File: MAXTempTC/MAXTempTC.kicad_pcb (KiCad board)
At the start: 2 copper layers, 15.6 x 29.1 mm, 12 parts, among them J1 1, J2 2, P5 OUTPUT, P6 INPUT, U3 MAX31855, U4 MAX31855

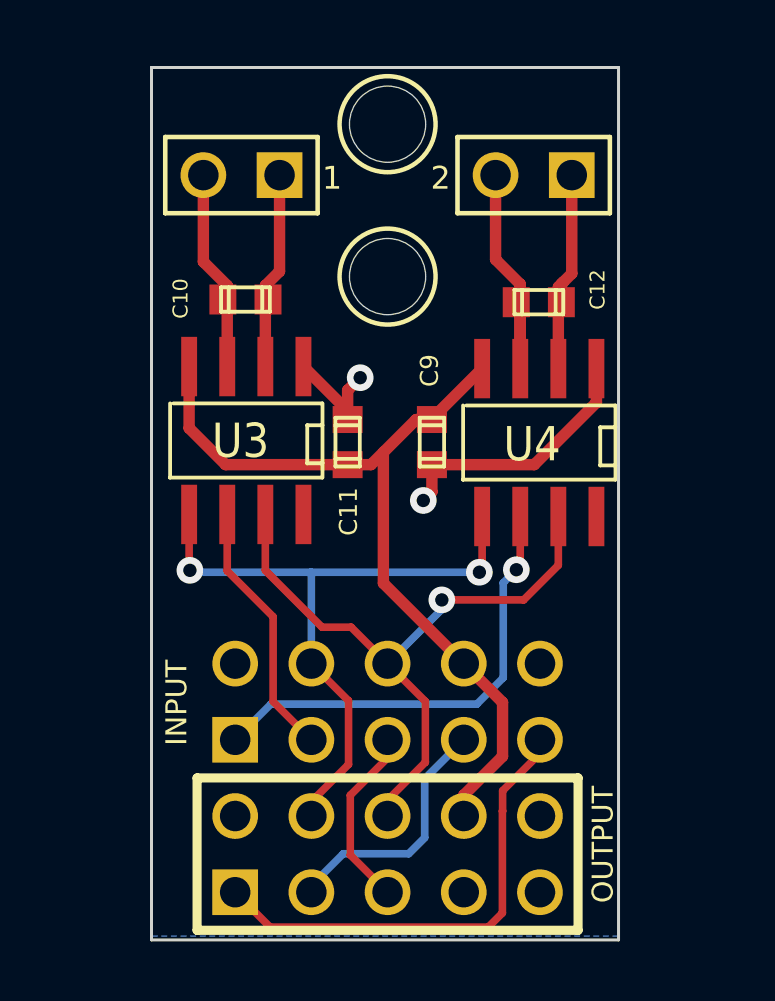
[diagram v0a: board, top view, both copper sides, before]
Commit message: Updated v1.1 source files
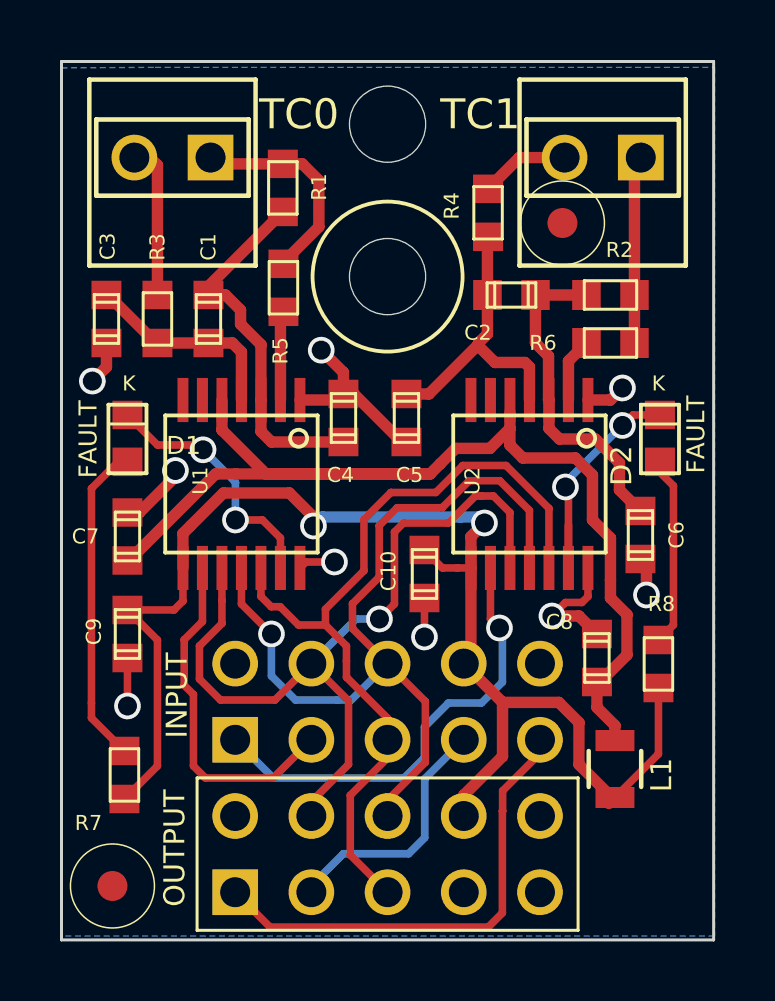
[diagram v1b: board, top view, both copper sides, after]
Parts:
- removed C11: 0.1u, c_0603
- removed C12: 0.01u, c_0603
- removed Mount (x2): VAL**, Mount
- removed U3, U4: MAX31855, MAX81855
- added C1: 0.1u, complib:C_0603, F.Cu at (43.4, 38.7)
- added C2: 0.1u, complib:C_0603, F.Cu at (53.5, 37.9)
- added C3: 0.01u, complib:C_0603, F.Cu at (40.0, 38.7)
- added C4: 0.01u, complib:C_0603, F.Cu at (47.9, 42.0)
- added C5: 0.01u, complib:C_0603, F.Cu at (50.0, 42.0)
- added C6: 0.01u, complib:C_0603, F.Cu at (57.8, 45.9)
- added C7: 0.1u, complib:C_0603, F.Cu at (40.7, 45.9)
- added C8: 0.1u, complib:C_0603, F.Cu at (56.4, 50.0)
- added D1: FAULT, complib:D_0603, F.Cu at (40.7, 42.7)
- added D2: FAULT, complib:D_0603, F.Cu at (58.5, 42.7)
- added G***: LOGO, complib:LOGO_Duet3dCompatible_xs, B.Cu at (42.8, 43.0)
- added L1: 100 µH, complib:R_0805, F.Cu at (57.0, 53.7)
- added M3: FID, complib:Fiducial_1mm_Dia_2.54mm_Outer_CopperTop, F.Cu at (40.2, 57.6)
- added M3: FID, complib:Fiducial_1mm_Dia_2.54mm_Outer_CopperTop, F.Cu at (55.2, 35.5)
- added R1: 100R, complib:R_0603, F.Cu at (45.9, 34.3)
- added R2: 100R, complib:R_0603, F.Cu at (56.8, 37.9)
- added R3: 100R, complib:R_0603, F.Cu at (41.7, 38.7)
- added R4: 100R, complib:R_0603, F.Cu at (52.8, 35.1)
- added R5: 100R, complib:R_0603, F.Cu at (45.9, 37.6)
- added R6: 100R, complib:R_0603, F.Cu at (56.8, 39.5)
- added R7: 330R, complib:R_0603, F.Cu at (40.6, 53.9)
- added R8: 330R, complib:R_0603, F.Cu at (58.4, 50.2)
- added U1: MAX31856, complib:TSSOP-14, F.Cu at (44.5, 44.2)
- added U2: MAX31856, complib:TSSOP-14, F.Cu at (54.1, 44.2)
- C10: value 0.01u -> 0.1u; footprint c_0603 -> complib:C_0603
- C9: footprint c_0603 -> complib:C_0603
- J1: value 1 -> ThermC1; footprint PIN_ARRAY_2X1 -> complib:PIN_ARRAY_2X1
- J2: value 2 -> ThermC2; footprint PIN_ARRAY_2X1 -> complib:PIN_ARRAY_2X1
- P5: footprint PIN_ARRAY_5x2 -> MAX_TEMP_DB
- P6: footprint PIN_ARRAY_5x2 -> complib:MAX_TEMP_DB_inv; moved to B.Cu
- moved C9 12.0 mm to (40.7, 49.2), turned to 270 degrees
- moved C10 10.9 mm to (50.6, 47.2), turned to 270 degrees
- moved J1 2.37 mm to (42.2, 33.3)
- moved J2 2.37 mm to (56.6, 33.3)
- turned P6 to 180 degrees
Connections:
- C10 pad 1: TC+_A -> AGND
- C10 pad 2: TC-_A -> 3.3V
- C9 pad 1: 3.3V -> AGND
- C9 pad 2: GND -> 3.3V
- P5 pad 2: GND -> AGND
- P6 pad 2: GND -> AGND
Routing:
- net AVDD: track 0.00 -> 37.5 mm
- net MOSI: track 6.13 -> 28.4 mm
- net AGND: track 0.00 -> 20.8 mm, vias 0 -> 9
- net 3.3V: track 28.0 -> 46.2 mm, vias 0 -> 2
- net GND: track 12.7 -> 0.00 mm, vias 2 -> 0
- net Net-(C1-Pad2): track 0.00 -> 12.3 mm
- net Net-(C2-Pad2): track 0.00 -> 11.1 mm
- net Net-(D1-Pad1): track 0.00 -> 10.8 mm
- net Net-(C2-Pad1): track 0.00 -> 10.0 mm
- net Net-(D1-Pad2): track 0.00 -> 8.54 mm, vias 0 -> 2
- net Net-(D2-Pad2): track 0.00 -> 8.42 mm, vias 0 -> 2
- net Net-(C1-Pad1): track 0.00 -> 6.89 mm
- net Net-(D2-Pad1): track 0.00 -> 6.48 mm
- net TC+_B: track 9.06 -> 2.98 mm
- net MISO: track 22.2 -> 28.3 mm
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- added copper zone on B.Cu, net AGND
- removed copper zone on B.Cu, net GND
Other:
- board size 15.6 x 29.1 mm -> 21.7 x 29.3 mm
- board text added: "MAXTempTC v1.1 Thermocouple Board By Think3dPrint3d and Escher3d CERN OHL v1.2 www.duet3d.com"
- board text added: "TC0"
- board text added: "TC1"
- board text removed: "MAXTempTC v0.2 K Thermocouple Board Design by: Think3dPrint3d Escher3d www.duet3d.com"
